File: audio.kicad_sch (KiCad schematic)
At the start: 26 parts, among them IC4 PCMD3180IRTWT

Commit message: New structure for holding parts, symbols, and footprints
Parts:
- CH1, CH2, CH3, CH4: footprint IM73D122V01XTMA1:PG-LLGA-5-2_INF -> CivicAlert:IM73D122V01XTMA1
- IC4: footprint PCMD3180IRTWR:QFN50P400X400X80-25N-D -> CivicAlert:PCMD3180IRTWT
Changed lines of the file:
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@@
 			)
 		)
-		(property "Footprint" "IM73D122V01XTMA1:PG-LLGA-5-2_INF"
+		(property "Footprint" "CivicAlert:IM73D122V01XTMA1"
 			(at 219.71 66.04 0)
 			(effects
@@
 			)
 		)
-		(property "Footprint" "PCMD3180IRTWR:QFN50P400X400X80-25N-D"
+		(property "Footprint" "CivicAlert:PCMD3180IRTWT"
 			(at 125.73 221.92 0)
 			(effects
@@
 			)
 		)
-		(property "Footprint" "IM73D122V01XTMA1:PG-LLGA-5-2_INF"
+		(property "Footprint" "CivicAlert:IM73D122V01XTMA1"
 			(at 125.73 66.04 0)
 			(effects
@@
 			)
 		)
-		(property "Footprint" "IM73D122V01XTMA1:PG-LLGA-5-2_INF"
+		(property "Footprint" "CivicAlert:IM73D122V01XTMA1"
 			(at 125.73 35.56 0)
 			(effects
@@
 			)
 		)
-		(property "Footprint" "IM73D122V01XTMA1:PG-LLGA-5-2_INF"
+		(property "Footprint" "CivicAlert:IM73D122V01XTMA1"
 			(at 219.71 35.56 0)
 			(effects

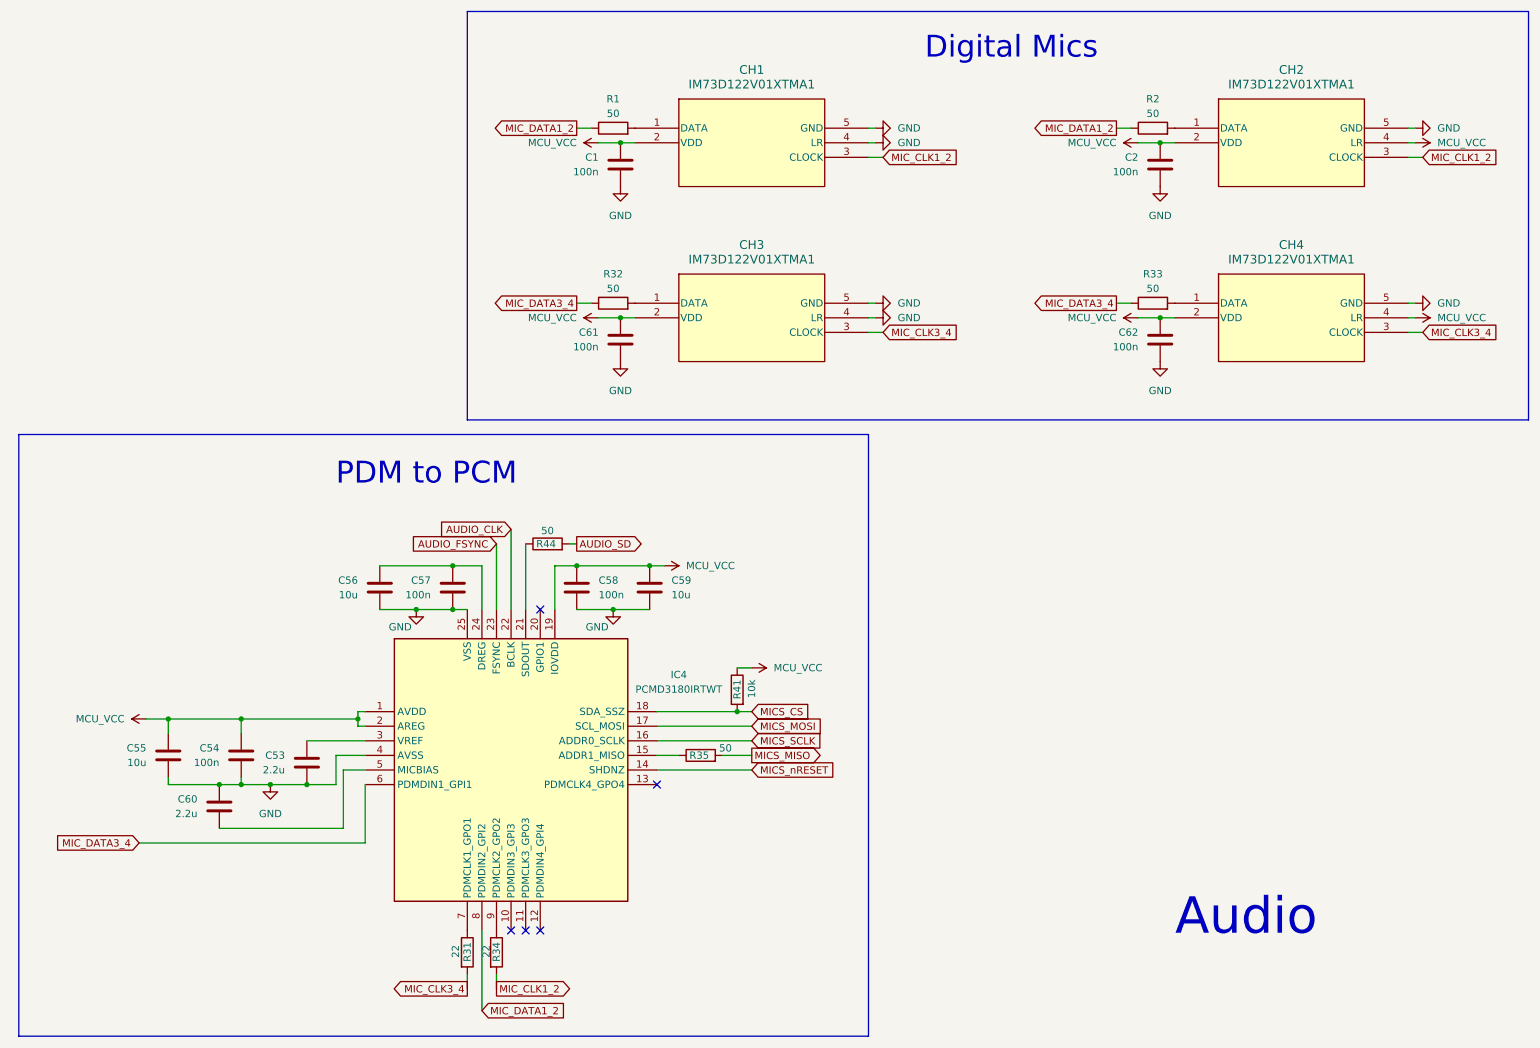
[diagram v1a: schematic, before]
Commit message: Update for RevB
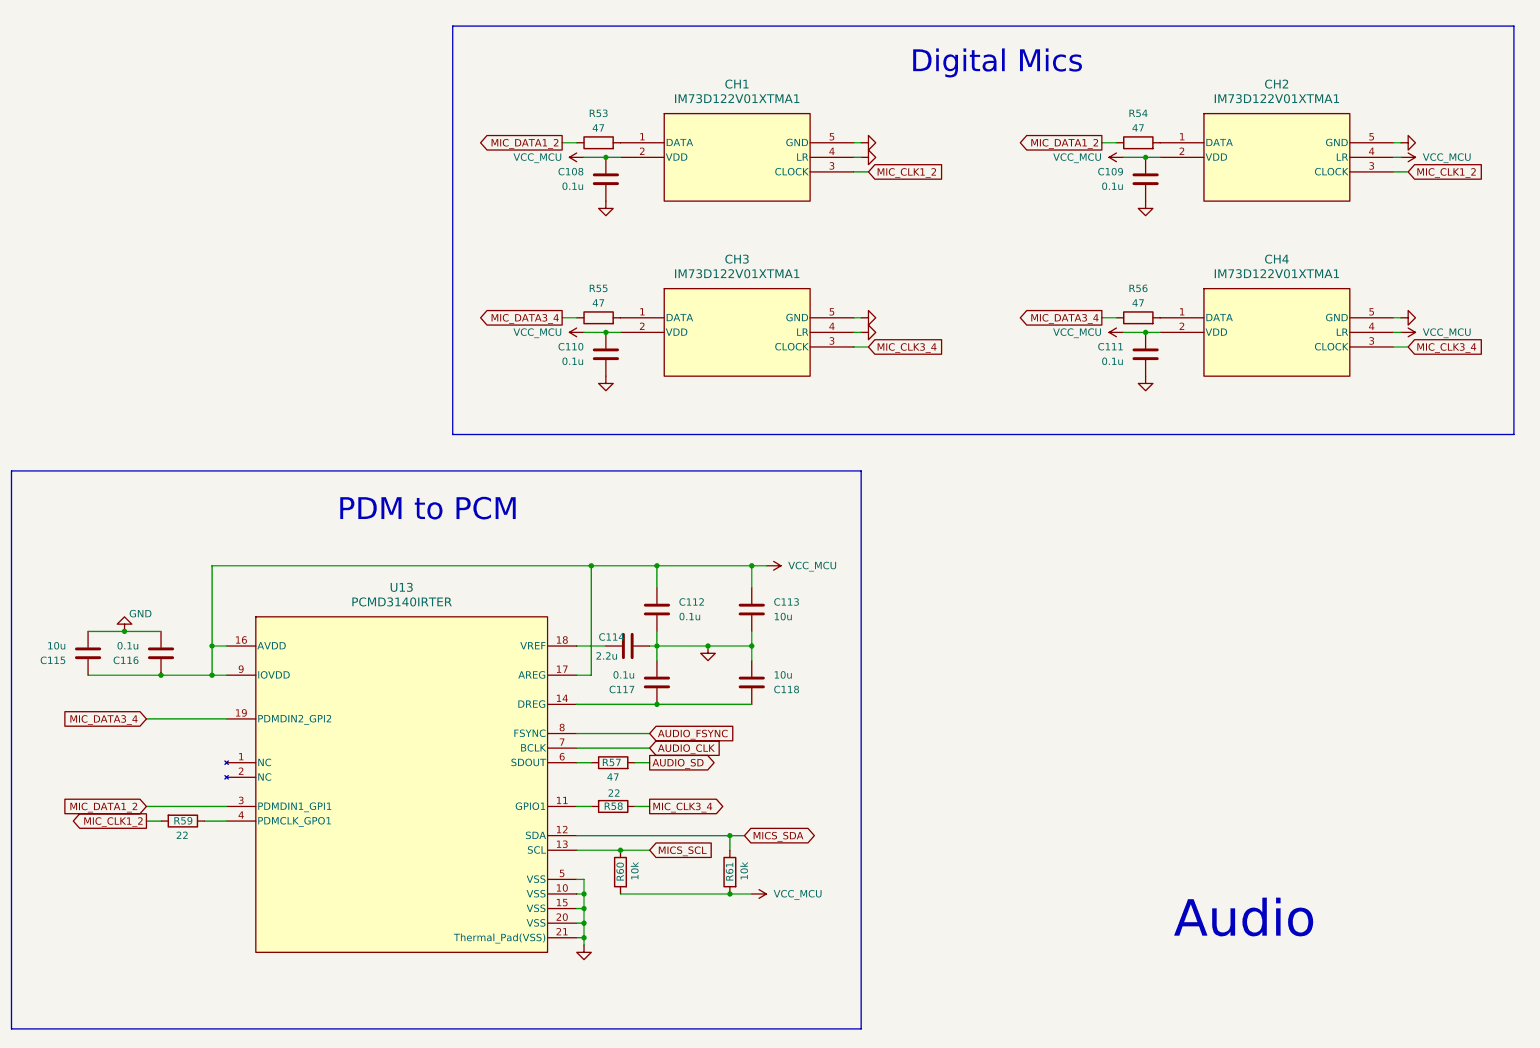
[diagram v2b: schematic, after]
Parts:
- removed C60: 2.2u, Capacitor_SMD:C_0402_1005Metric, symbol Device:C
- removed IC4: PCMD3180IRTWT, CivicAlert:PCMD3180IRTWT, symbol PCMD3180IRTWT:PCMD3180IRTWT
- removed R35: 50, Resistor_SMD:R_0402_1005Metric, symbol Device:R
- added R61: 10k, Resistor_SMD:R_0402_1005Metric, symbol Device:R
- added U13: PCMD3140IRTER, CivicAlert:PCMD3140IRTER, symbol PCMD3140IRTER:PCMD3140IRTER
- C108: renamed from C1; value 100n -> 0.1u; MANUFACTURER Murata -> (none); MPN GRT155R71H104KE01D -> (none); Manufacturer (none) -> Murata
- C109: renamed from C2; value 100n -> 0.1u; MANUFACTURER Murata -> (none); MPN GRT155R71H104KE01D -> (none); Manufacturer (none) -> Murata
- C110: renamed from C61; value 100n -> 0.1u; MANUFACTURER Murata -> (none); MPN GRT155R71H104KE01D -> (none); Manufacturer (none) -> Murata
- C111: renamed from C62; value 100n -> 0.1u; MANUFACTURER Murata -> (none); MPN GRT155R71H104KE01D -> (none); Manufacturer (none) -> Murata
- C112: renamed from C54; value 100n -> 0.1u; MANUFACTURER Murata -> (none); MPN GRT155R71H104KE01D -> (none); Manufacturer (none) -> Murata
- C113: renamed from C55; footprint Capacitor_SMD:C_0402_1005Metric -> Capacitor_SMD:C_0603_1608Metric; MANUFACTURER Murata -> (none); MPN GRT155R61A106ME13J -> (none); Manufacturer (none) -> Murata
- C114: renamed from C53; MANUFACTURER Murata -> (none); MPN GRT155C71A225KE13D -> (none); Manufacturer (none) -> Murata
- C115: renamed from C59; footprint Capacitor_SMD:C_0402_1005Metric -> Capacitor_SMD:C_0603_1608Metric; MANUFACTURER Murata -> (none); MPN GRT155R61A106ME13J -> (none); Manufacturer (none) -> Murata
- C116: renamed from C58; value 100n -> 0.1u; MANUFACTURER Murata -> (none); MPN GRT155R71H104KE01D -> (none); Manufacturer (none) -> Murata
- C117: renamed from C57; value 100n -> 0.1u; MANUFACTURER Murata -> (none); MPN GRT155R71H104KE01D -> (none); Manufacturer (none) -> Murata
- C118: renamed from C56; footprint Capacitor_SMD:C_0402_1005Metric -> Capacitor_SMD:C_0603_1608Metric; MANUFACTURER Murata -> (none); MPN GRT155R61A106ME13J -> (none); Manufacturer (none) -> Murata
- CH1, CH2, CH3, CH4: MANUFACTURER Infineon -> (none); MPN IM73D122V01XTMA1 -> (none); Manufacturer (none) -> Infineon
- R53: renamed from R1; value 50 -> 47
- R54: renamed from R2; value 50 -> 47
- R55: renamed from R32; value 50 -> 47
- R56: renamed from R33; value 50 -> 47
- R57: renamed from R44; value 50 -> 47
- renumbered R34 to R58, R31 to R59, R41 to R60
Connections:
- net MICS_CS is gone; now on net VCC_MCU: R60.2
- net AUDIO_CLK: now also U13.7 (BCLK)
- net AUDIO_FSYNC: now also U13.8 (FSYNC)
- net GND: now also U13.10 (VSS), U13.15 (VSS), U13.20 (VSS), U13.21 (Thermal_Pad(VSS)), U13.5 (VSS)
- net MIC_CLK1_2: now also R59.2; no longer R58.2
- net MIC_CLK3_4: now also R58.1; no longer R59.2
- net MIC_DATA1_2: now also U13.3 (PDMDIN1_GPI1)
- net MIC_DATA3_4: now also U13.19 (PDMDIN2_GPI2)
- net at R57.1: now also U13.6 (SDOUT)
- net at C117.1, C118.1: now also U13.14 (DREG)
- net at C114.1: now also U13.18 (VREF)
- net at R59.1: now also U13.4 (PDMCLK_GPO1)
- net MCU_VCC renamed VCC_MCU
- net VCC_MCU: now also R61.2, U13.16 (AVDD), U13.17 (AREG), U13.9 (IOVDD); no longer R60.1
- new net: R58.2, U13.11 (GPIO1)
- new net MICS_SCL: R60.1, U13.13 (SCL)
- new net MICS_SDA: R61.1, U13.12 (SDA)
- no-connect marks 5 -> 0
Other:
- moved on the sheet: C108, C109, C110, C111, C112, C113, C114, C115, C116, C117, C118, CH1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
